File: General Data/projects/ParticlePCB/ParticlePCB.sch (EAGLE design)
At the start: 11 parts, among them X1 RJ45-6L-B

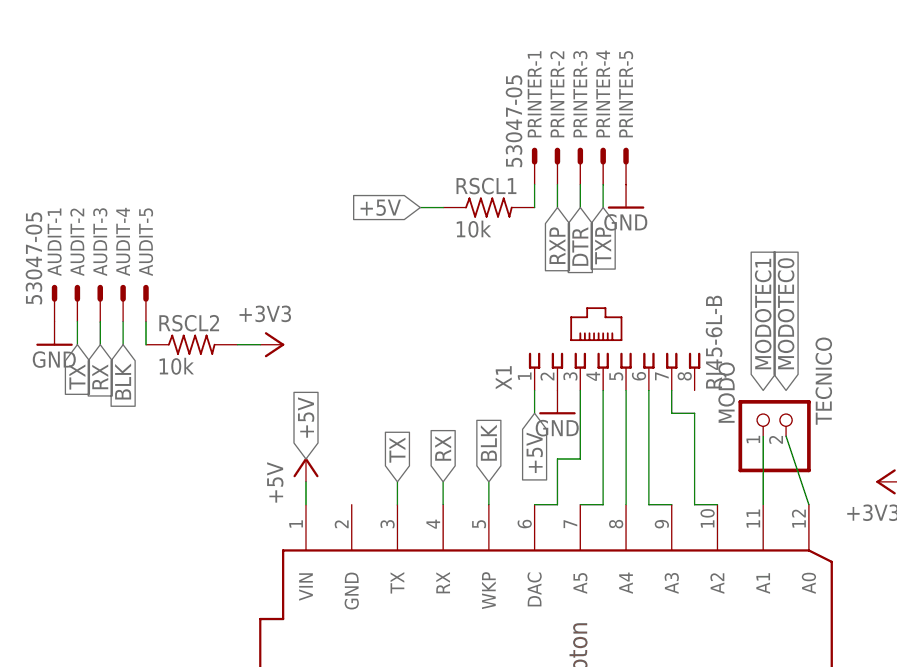
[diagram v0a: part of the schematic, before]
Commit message: Actualización de PCBs
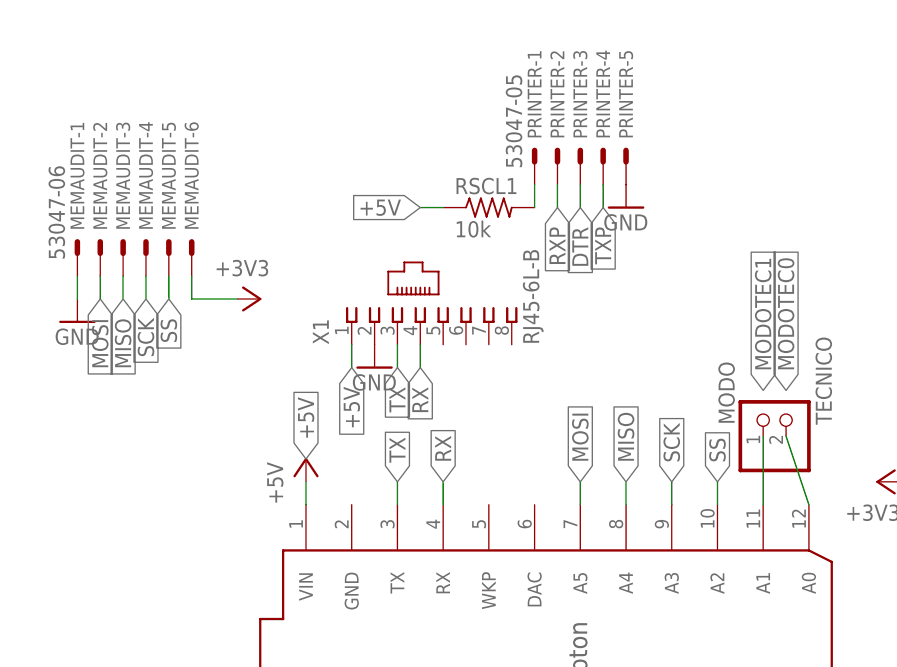
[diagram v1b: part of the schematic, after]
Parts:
- removed AUDIT: 53047-05, PNP:53047-05
- removed RSCL2: 10k, rcl:R-US_0207/10
- added MEMAUDIT: 53047-06, PNP:53047-06
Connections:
- removed net BLK: AUDIT-4.S, U$2.WKP
- removed net N$2: AUDIT-5.S, RSCL2.1
- removed net N$3: U$2.DAC, X1.3
- removed net N$4: U$2.A5, X1.4
- removed net N$5: U$2.A4, X1.5
- removed net N$6: U$2.A3, X1.6
- removed net N$7: U$2.A2, X1.7
- new net MISO: MEMAUDIT-3.S, U$2.A4
- new net MOSI: MEMAUDIT-2.S, U$2.A5
- new net SCK: MEMAUDIT-4.S, U$2.A3
- new net SS: MEMAUDIT-5.S, U$2.A2
- net +3V3: now also MEMAUDIT-6.S; no longer RSCL2.2
- net GND: now also MEMAUDIT-1.S; no longer AUDIT-1.S
- net RX: now also X1.4; no longer AUDIT-3.S
- net TX: now also X1.3; no longer AUDIT-2.S
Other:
- moved on the sheet: X1
